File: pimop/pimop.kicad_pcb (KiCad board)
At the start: 2 copper layers, 69 x 80.8 mm, 12 parts, among them U1 FR232rl, con1 pmod_12, con2 pmod_12, con3 pmod_12, con4 usb-c, j1 pinheader, sw1 switch

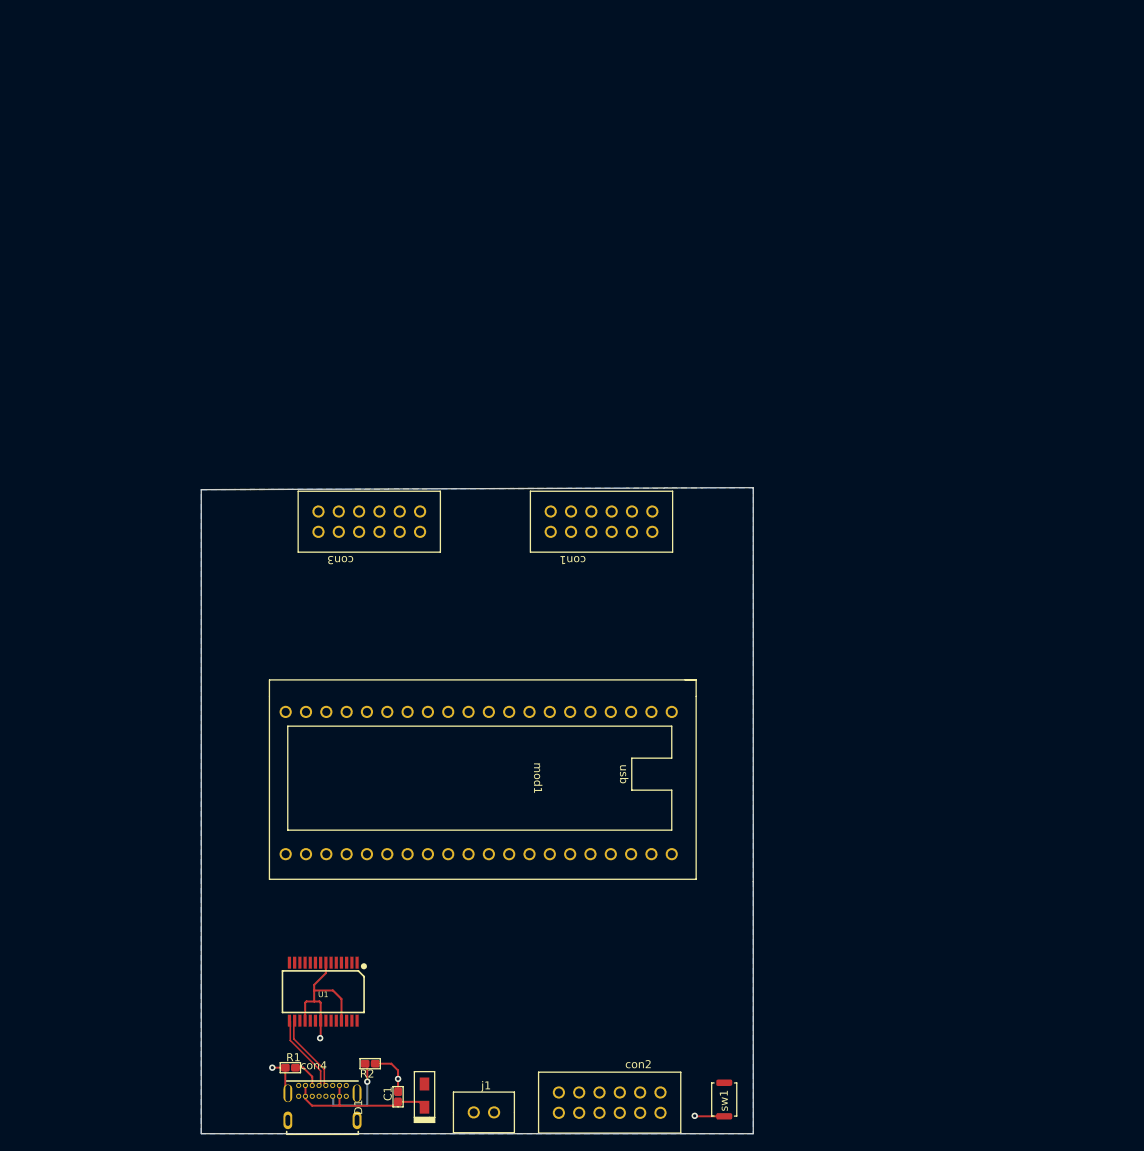
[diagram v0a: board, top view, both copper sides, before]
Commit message: e5yt
45y
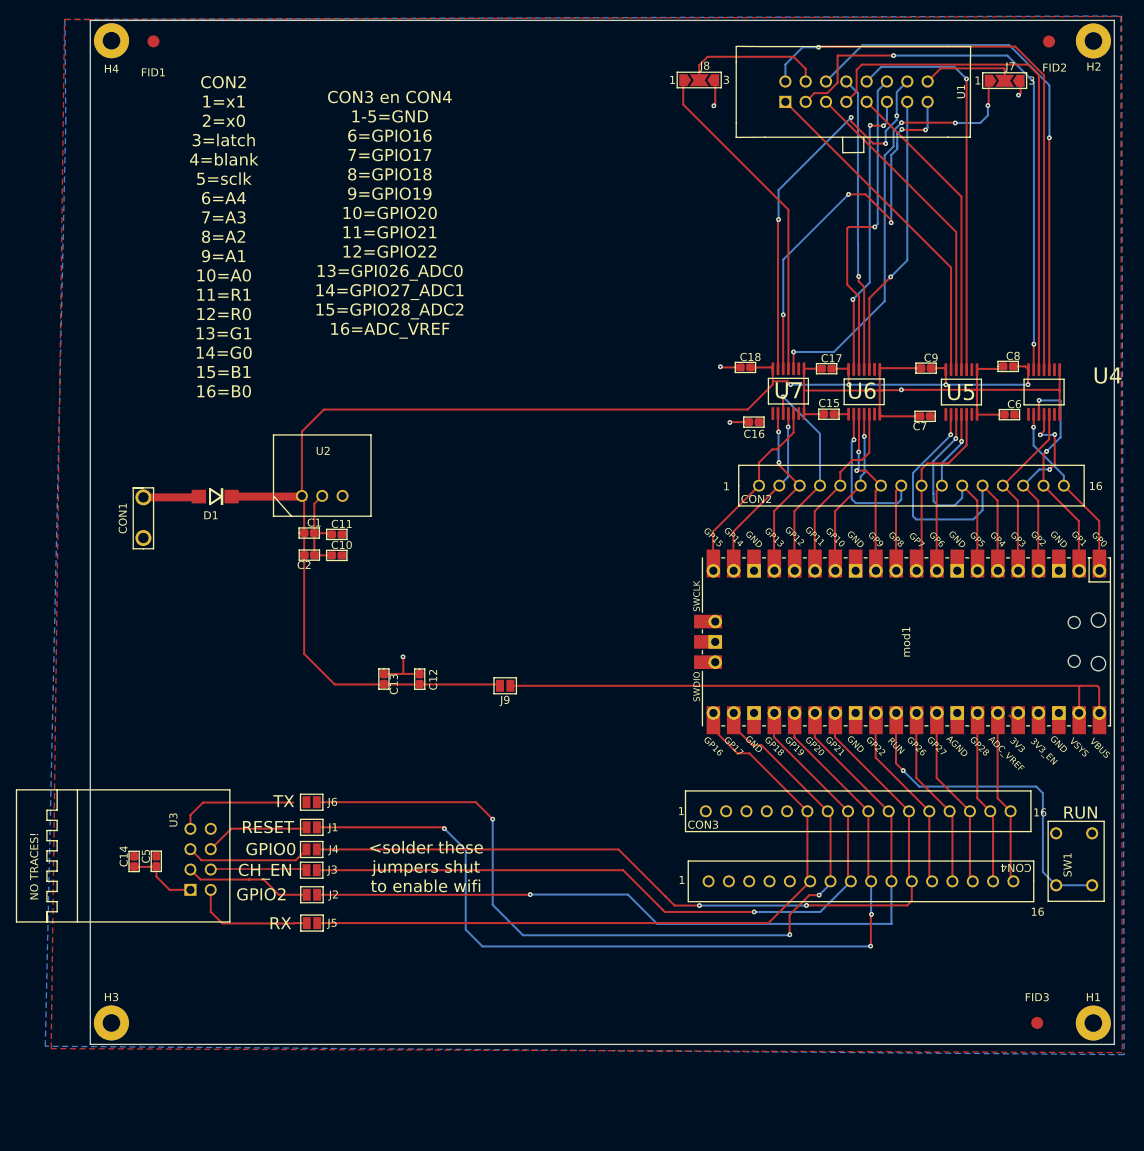
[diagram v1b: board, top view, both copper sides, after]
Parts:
- removed R1, R2: resistor, vanalles:0603RL
- removed con1, con2, con3: pmod_12, connectors_user:PMOD12
- removed con4: usb-c, connectors_user:GCT_USB4085-GF-A_REVA
- removed j1: pinheader, connectors_user:heaer2pin
- removed sw1: switch, vanalles:Alps_SKRK
- added C10: 10uF, vanalles:0603, F.Cu at (108.5, 92.4)
- added C11: 100nF, vanalles:0603, F.Cu at (108.5, 89.8)
- added C12: 10uF, vanalles:0603, F.Cu at (118.8, 107.9)
- added C13: 100nF, vanalles:0603, F.Cu at (114.4, 107.9)
- added C14: 100nF, vanalles:0603, F.Cu at (83.1, 130.7)
- added C15: 10uF, vanalles:0603, F.Cu at (170.0, 74.7)
- added C16: 10uF, vanalles:0603, F.Cu at (160.6, 75.7)
- added C17: 10uF, vanalles:0603, F.Cu at (169.7, 69.1)
- added C18: 10uF, vanalles:0603, F.Cu at (159.6, 68.9)
- added C2: 100nF, vanalles:0603, F.Cu at (105.0, 92.4)
- added C5: 10uF, vanalles:0603, F.Cu at (85.9, 130.6)
- added C6: 10uF, vanalles:0603, F.Cu at (192.6, 74.8)
- added C7: 10uF, vanalles:0603, F.Cu at (182.0, 75.0)
- added C8: 10uF, vanalles:0603, F.Cu at (192.4, 68.8)
- added C9: 10uF, vanalles:0603, F.Cu at (182.1, 69.0)
- added CON1: con_2pin, connectors_user:2pin_screw_vast, F.Cu at (84.3, 87.8)
- added CON2: 16pinheader, connectors_user:16 pin, F.Cu at (179.0, 83.7)
- added CON3: 16pinheader, connectors_user:16 pin, F.Cu at (172.4, 124.4)
- added CON4: 16pinheader, connectors_user:16 pin, F.Cu at (175.3, 133.1)
- added FID1: Fiducial, vanalles:Fiducial_1.5mm_Mask4.5mm, F.Cu at (85.6, 28.1)
- added FID2: Fiducial, vanalles:Fiducial_1.5mm_Mask4.5mm, F.Cu at (197.5, 28.2)
- added FID3: Fiducial, vanalles:Fiducial_1.5mm_Mask4.5mm, F.Cu at (196.0, 150.8)
- added H1: MountingHole, vanalles:MountingHole_2.2mm_M2_Pad, F.Cu at (203.0, 150.9)
- added H2: MountingHole, vanalles:MountingHole_2.2mm_M2_Pad, F.Cu at (203.1, 28.1)
- added H3: MountingHole, vanalles:MountingHole_2.2mm_M2_Pad, F.Cu at (80.3, 150.8)
- added H4: MountingHole, vanalles:MountingHole_2.2mm_M2_Pad, F.Cu at (80.3, 28.1)
- added J1: solderjumper_2pin, vanalles:SolderJumper-2_P1.3mm_Open_Pad1.0x1.5mm, F.Cu at (105.3, 126.4)
- added J2: solderjumper_2pin, vanalles:SolderJumper-2_P1.3mm_Open_Pad1.0x1.5mm, F.Cu at (105.4, 134.8)
- added J3: solderjumper_2pin, vanalles:SolderJumper-2_P1.3mm_Open_Pad1.0x1.5mm, F.Cu at (105.3, 131.8)
- added J4: solderjumper_2pin, vanalles:SolderJumper-2_P1.3mm_Open_Pad1.0x1.5mm, F.Cu at (105.3, 129.2)
- added J5: solderjumper_2pin, vanalles:SolderJumper-2_P1.3mm_Open_Pad1.0x1.5mm, F.Cu at (105.4, 138.4)
- added J6: solderjumper_2pin, vanalles:SolderJumper-2_P1.3mm_Open_Pad1.0x1.5mm, F.Cu at (105.3, 123.2)
- added J7: solder_jumper3, vanalles:SolderJumper-3_P2.0mm_Open_TrianglePad1.0x1.5mm_NumberLabels, F.Cu at (191.9, 33.1)
- added J8: solder_jumper3, vanalles:SolderJumper-3_P2.0mm_Open_TrianglePad1.0x1.5mm_NumberLabels, F.Cu at (153.8, 33.0)
- added J9: solderjumper_2pin, vanalles:SolderJumper-2_P1.3mm_Open_Pad1.0x1.5mm, F.Cu at (129.5, 108.7)
- added SW1: button, vanalles:button, F.Cu at (200.9, 130.6)
- added U2: recom_psu, vanalles:recom psu, F.Cu at (106.7, 85.0)
- added U3: esp8266_mod1, Module:esp8266mod, F.Cu at (81.8, 130.0)
- added U4: TXB0104, halfgeleiders:Texas_TXB0104PWR, F.Cu at (196.9, 72.0)
- added U5: TXB0104, halfgeleiders:Texas_TXB0104PWR, F.Cu at (186.6, 72.0)
- added U6: TXB0104, halfgeleiders:Texas_TXB0104PWR, F.Cu at (174.4, 72.0)
- added U7: TXB0104, halfgeleiders:Texas_TXB0104PWR, F.Cu at (164.9, 71.9)
- C1: value 47u -> 10uF; footprint vanalles:0603RL -> vanalles:0603
- D1: value MBR120 -> Diode; footprint halfgeleiders:SOD123 -> halfgeleiders:DO214
- U1: value FR232rl -> Led_Pannel; footprint halfgeleiders:SSOP28-0.65-10.2X5.2MM -> connectors_user:2x8
- mod1: value rpi_pico -> picorpi; footprint Module:rpi pico -> Module:RPi_Pico_SMD_TH
- moved U1 130.5 mm to (173.0, 34.5), turned to 90 degrees
- moved D1 80.7 mm to (93.3, 85.0), turned to 180 degrees
- moved C1 72.0 mm to (105.0, 89.6), turned to 0 degrees
- moved mod1 52.0 mm to (179.7, 103.2)
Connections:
- net Net-(C1-Pad1) renamed +5V
- D1 pad 1: /VSYS -> Net-(CON1-Pad2)
- U1 pad 1: /TX -> /ledpannel/R0_IL
- U1 pad 10: no_connect_38 -> /ledpannel/A1_IL
- U1 pad 11: no_connect_39 -> /ledpannel/A2_IL
- U1 pad 12: no_connect_40 -> /ledpannel/A3_IL
- U1 pad 13: no_connect_41 -> /ledpannel/SCLK_IL
- U1 pad 14: no_connect_42 -> /ledpannel/LATCH_IL
- U1 pad 15: /D_P -> /ledpannel/BLANK_IL
- U1 pad 16: /D_N -> Net-(J7-Pad2)
- U1 pad 2: no_connect_45 -> /ledpannel/G0_IL
- U1 pad 3: no_connect_51 -> /ledpannel/B0_IL
- U1 pad 4: +3V3 -> Net-(J8-Pad2)
- U1 pad 5: /RX -> /ledpannel/R1_IL
- U1 pad 6: no_connect_52 -> /ledpannel/G1_IL
- U1 pad 7: GND -> /ledpannel/B1_IL
- U1 pad 8: (no net) -> /ledpannel/A4_IL
- U1 pad 9: no_connect_53 -> /ledpannel/A0_IL
- mod1 pad 1: /GP0 -> /level shifters/B0_IL
- mod1 pad 10: /GP7 -> /level shifters/A1_IL
- mod1 pad 11: /GP8 -> /level shifters/A2_IL
- mod1 pad 12: /GP9 -> /level shifters/A3_IL
- mod1 pad 14: /GP10 -> /level shifters/A4_IL
- mod1 pad 15: /GP11 -> /level shifters/SCLK_IL
- mod1 pad 16: /GP12 -> /level shifters/BLANK_IL
- mod1 pad 17: /GP13 -> /rpi pico/LATCH
- mod1 pad 19: /GP14 -> /level shifters/X0_IL
- mod1 pad 2: /GP1 -> /level shifters/B1_IL
- mod1 pad 20: /GP15 -> /level shifters/X1_IL
- mod1 pad 21: /TX -> /rpi pico/GPIO16
- mod1 pad 22: /RX -> /rpi pico/GPIO17
- mod1 pad 24: /GP18 -> /rpi pico/GPIO18
- mod1 pad 25: /GP19 -> /rpi pico/GPIO19
- mod1 pad 26: /GP20 -> /rpi pico/GPIO20
- mod1 pad 27: /GP21 -> /rpi pico/GPIO21
- mod1 pad 29: /GP22 -> /rpi pico/GPIO22
- mod1 pad 30: /RUN -> Net-(SW1-Pad1)
- mod1 pad 31: /GP26 -> /rpi pico/GPIO26_ADC0
- mod1 pad 32: /GP27 -> /rpi pico/GPIO27_ADC1
- mod1 pad 34: /GP28 -> /rpi pico/GPIO28_ADC2
- mod1 pad 35: no_connect_56 -> /rpi pico/ADC_VREF
- mod1 pad 37: no_connect_57 -> unconnected-(mod1-Pad37)
- mod1 pad 39: /VSYS -> Net-(mod1-Pad39)
- mod1 pad 4: /GP2 -> /rpi pico/G0
- mod1 pad 40: VBUS -> Net-(mod1-Pad39)
- mod1 pad 5: /GP3 -> /rpi pico/G1
- mod1 pad 6: /GP4 -> /rpi pico/R0
- mod1 pad 7: /GP5 -> /level shifters/R1_IL
- mod1 pad 9: /GP6 -> /level shifters/A0_IL
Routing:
- net +5V: track 20.0 -> 174.1 mm, vias 0 -> 4
- net /rpi pico/GPIO19: track 0.00 -> 114.3 mm, vias 0 -> 3
- net /rpi pico/GPIO17: track 0.00 -> 108.5 mm, vias 0 -> 3
- net /rpi pico/GPIO21: track 0.00 -> 104.9 mm, vias 0 -> 2
- net /rpi pico/GPIO20: track 0.00 -> 103.6 mm, vias 0 -> 1
- net /rpi pico/GPIO18: track 0.00 -> 95.4 mm, vias 0 -> 1
- net /rpi pico/GPIO16: track 0.00 -> 90.6 mm
- net GND: track 35.4 -> 115.8 mm, vias 4 -> 6
- net Net-(mod1-Pad39): track 0.00 -> 80.4 mm
- net /ledpannel/G0_IL: track 0.00 -> 73.7 mm, vias 0 -> 1
- net /ledpannel/B0_IL: track 0.00 -> 70.2 mm, vias 0 -> 2
- net /ledpannel/G1_IL: track 0.00 -> 67.4 mm, vias 0 -> 1
- net /ledpannel/B1_IL: track 0.00 -> 64.9 mm
- net /ledpannel/X1_IL: track 0.00 -> 54.9 mm, vias 0 -> 4
- net /ledpannel/BLANK_IL: track 0.00 -> 51.7 mm, vias 0 -> 5
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- added copper zone on F.Cu, net +3V3
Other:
- board size 69 x 80.8 mm -> 128 x 128 mm
- board text added: "1"
- board text added: "16"
- board text added: "<solder these jumpers shut to enable wifi"
- board text added: "CH_EN"
- board text added: "CON2 1=x1 2=x0 3=latch 4=blank 5=sclk 6=A4 7=A3 8=A2 9=A1 10=A0 11=R1 12=R0 13=G1 14=G0 15=B1 16=B0"
- board text added: "CON3 en CON4 1-5=GND 6=GPIO16 7=GPIO17 8=GPIO18 9=GPIO19 10=GPIO20 11=GPIO21 12=GPIO22 13=GPI026_ADC0 14=GPIO27_ADC1 15=GPIO28_ADC2 16=ADC_VREF"
- board text added: "GPIO0"
- board text added: "GPIO2"
- board text added: "RESET"
- board text added: "RUN"
- board text added: "RX"
- board text added: "TX"
